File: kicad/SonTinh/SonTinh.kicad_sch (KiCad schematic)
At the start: 11 parts, among them J10 1985195, J11 Conn_01x03_Socket, J12 1985195, J13 Conn_01x03_Socket, J3 Conn_02x03_Odd_Even, J4 1985218, J5 1985218, J7 1985195, J8 1985195

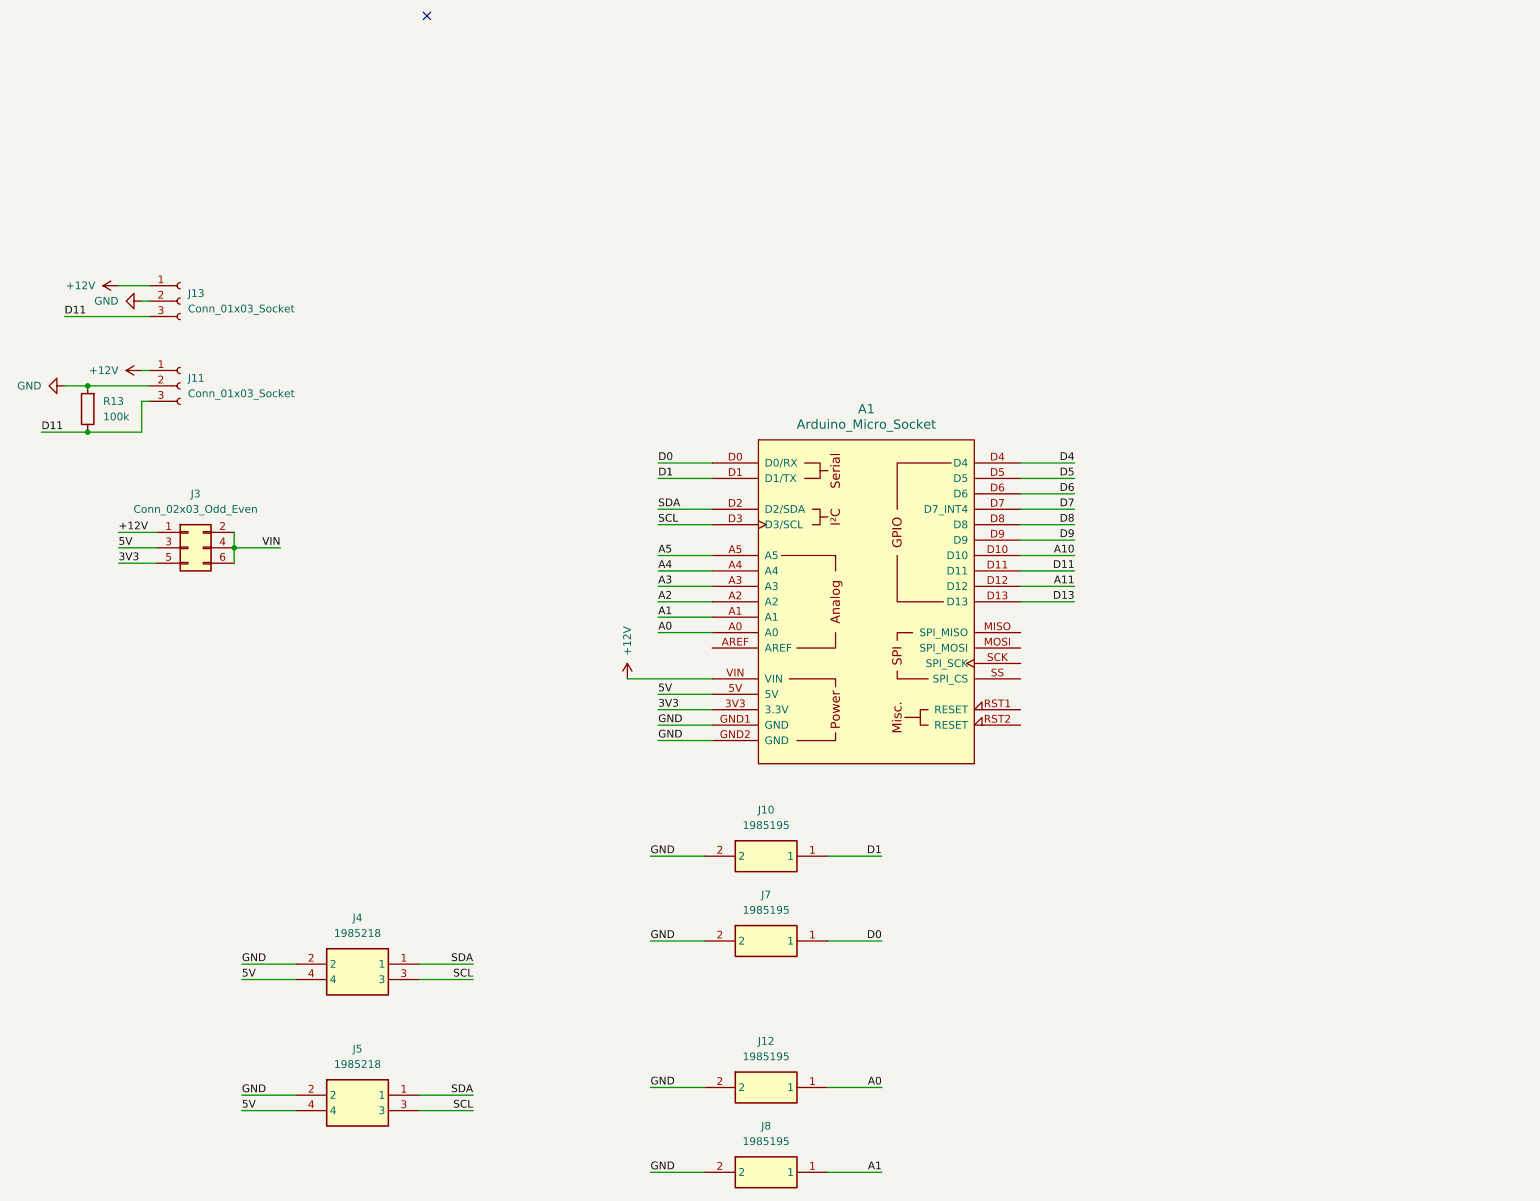
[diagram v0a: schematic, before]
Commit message: The Quill Is Mightier…
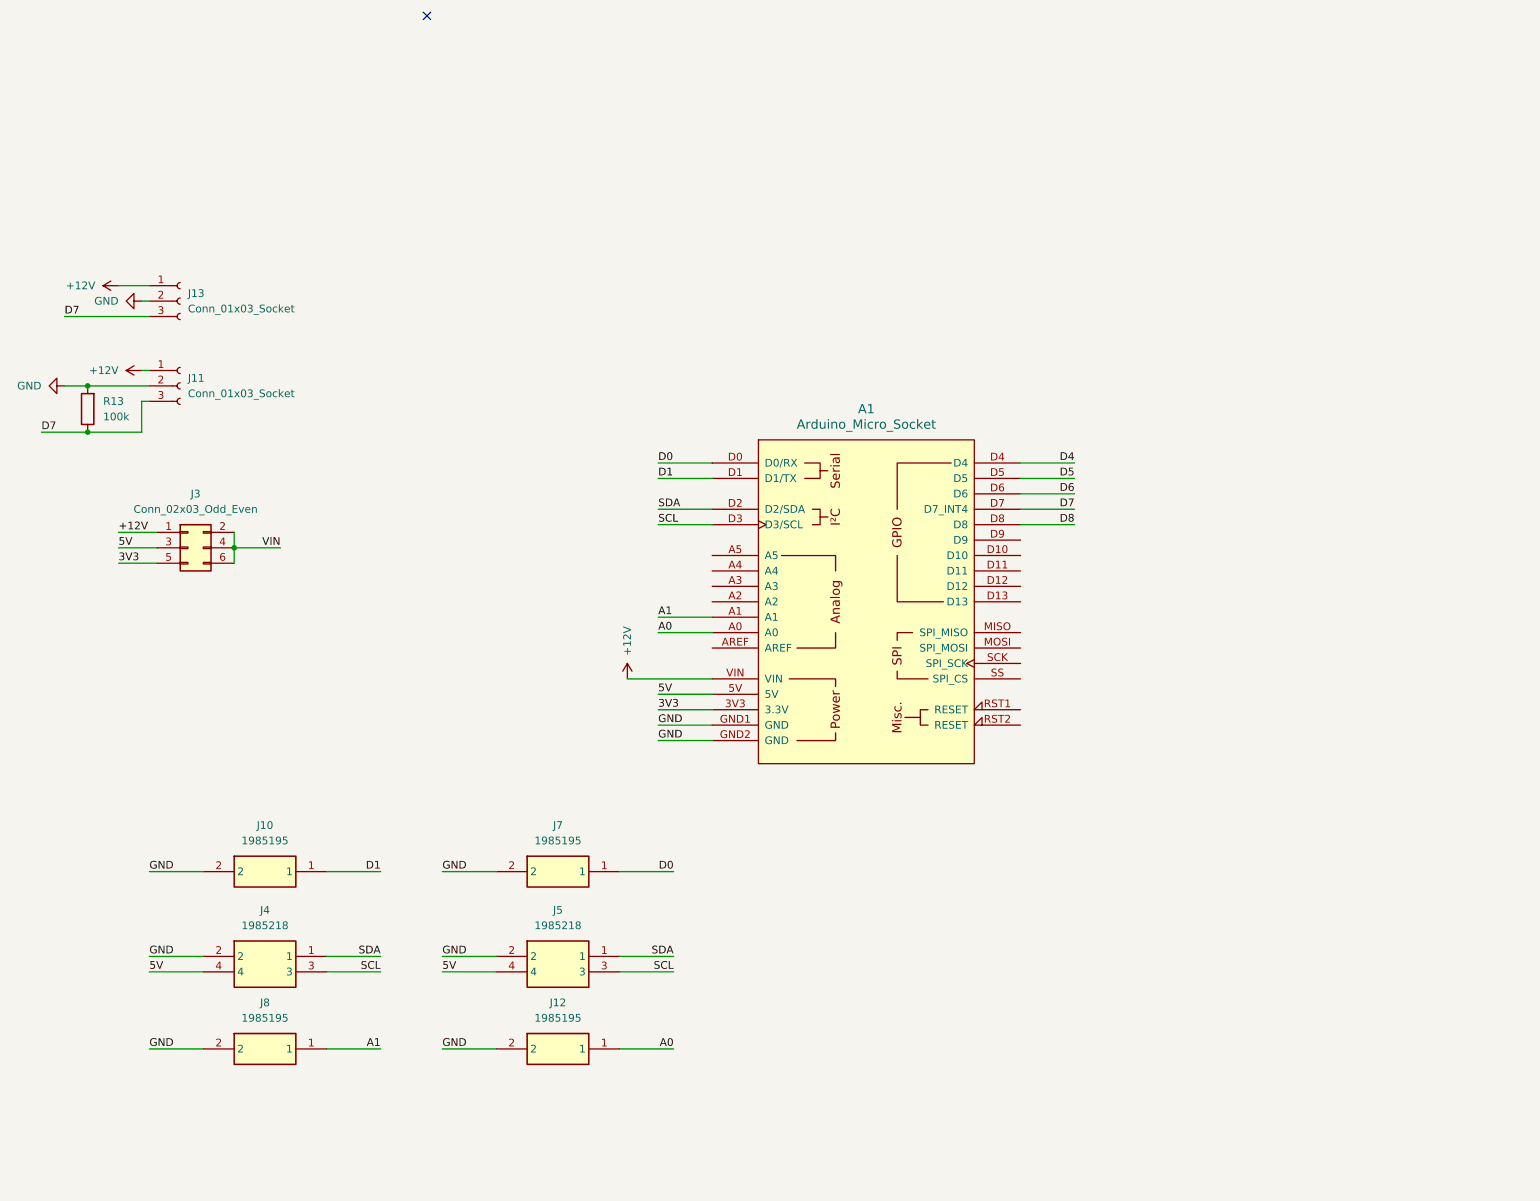
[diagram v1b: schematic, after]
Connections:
- net D7: now also J11.3 (Pin_3), J13.3 (Pin_3), R13.1
- net A10: no longer names the net of A1.D10
- net A11: no longer names the net of A1.D12
- net A2: no longer names the net of A1.A2
- net A3: no longer names the net of A1.A3
- net A4: no longer names the net of A1.A4
- net A5: no longer names the net of A1.A5
- removed net D11: A1.D11, J11.3 (Pin_3), J13.3 (Pin_3), R13.1
- net D13: no longer names the net of A1.D13
- net D9: no longer names the net of A1.D9
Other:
- moved on the sheet: J10, J12, J4, J5, J7, J8

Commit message: The Bitter Suite
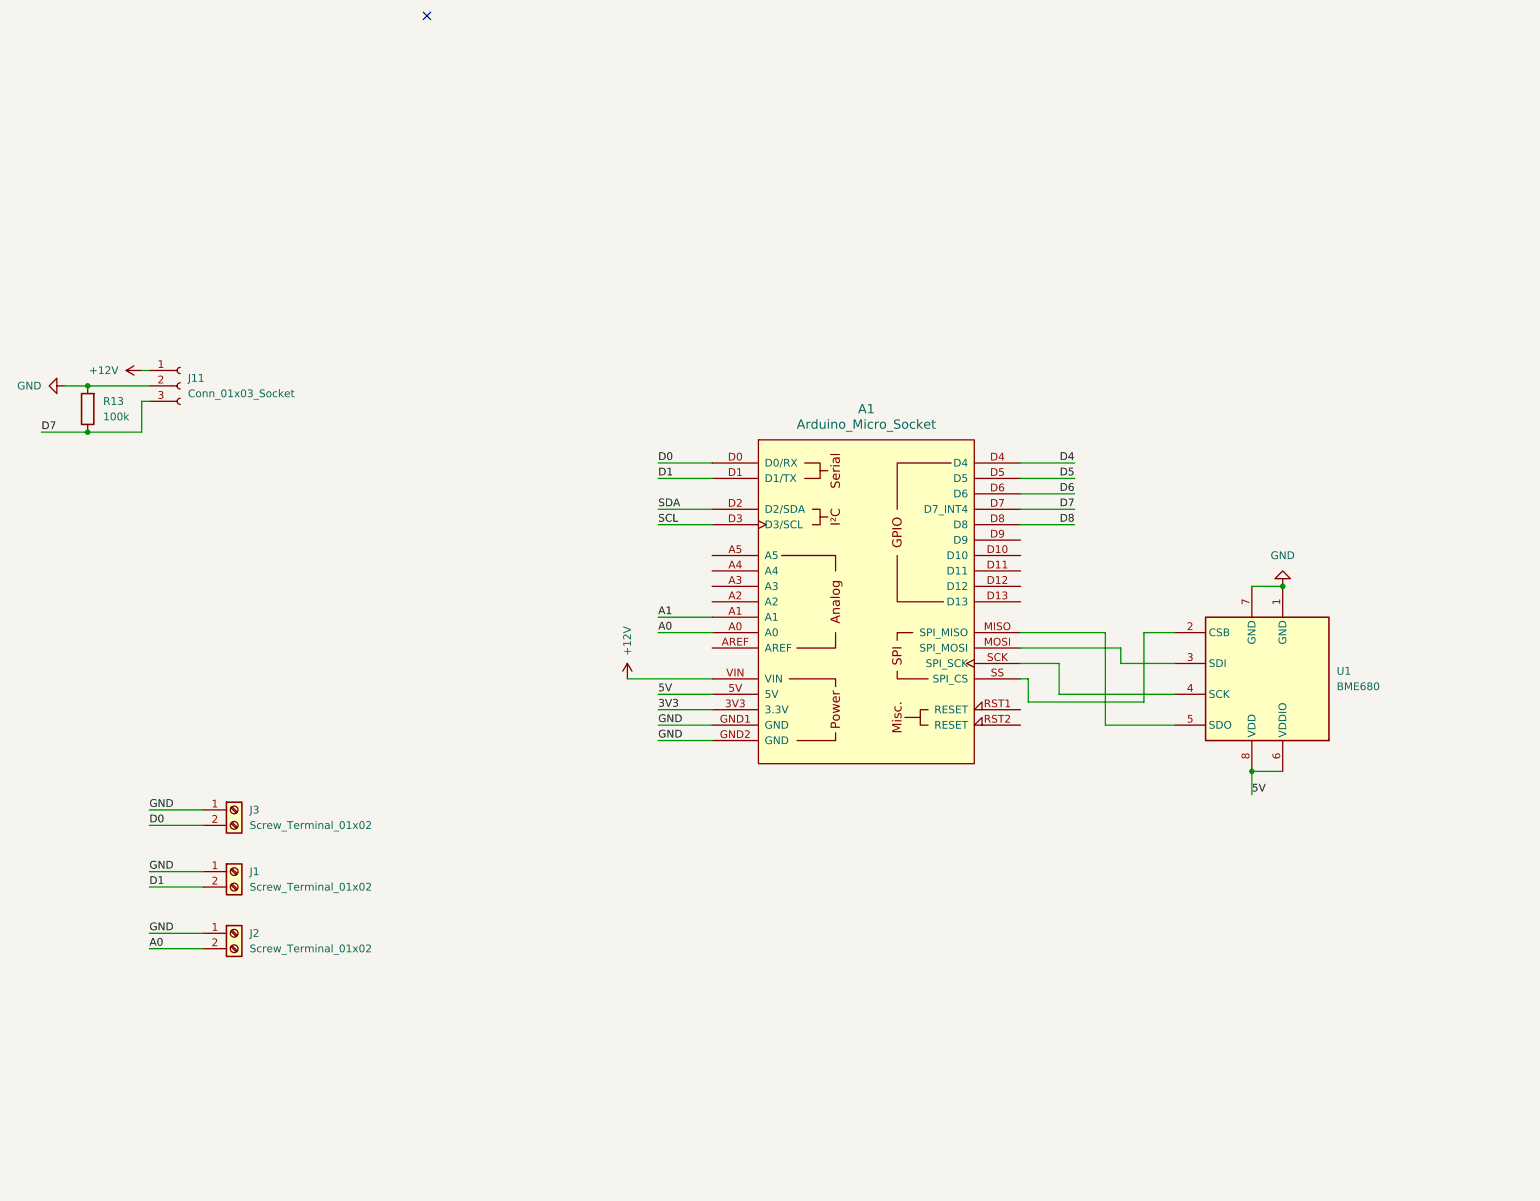
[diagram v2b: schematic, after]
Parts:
- removed J10, J12, J7, J8: 1985195, footprints:1985195, symbol PheonixContact:1985195
- removed J13: Conn_01x03_Socket, Connector_Wire:SolderWire-0.25sqmm_1x03_P4.5mm_D0.65mm_OD2mm, symbol Connector:Conn_01x03_Socket
- removed J3: Conn_02x03_Odd_Even, Connector_PinHeader_2.54mm:PinHeader_2x03_P2.54mm_Vertical, symbol Connector_Generic:Conn_02x03_Odd_Even
- removed J4, J5: 1985218, footprints:PTSA_15_4_35_Z, symbol PheonixContact:1985218
- added J1, J2, J3: Screw_Terminal_01x02, TerminalBlock_Phoenix:TerminalBlock_Phoenix_MPT-0,5-2-2.54_1x02_P2.54mm_Horizontal, symbol Connector:Screw_Terminal_01x02
- added U1: BME680, Package_LGA:Bosch_LGA-8_3x3mm_P0.8mm_ClockwisePinNumbering, symbol Sensor:BME680
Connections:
- net 5V: now also U1.6 (VDDIO), U1.8 (VDD)
- net A0: now also J2.2 (Pin_2)
- net D0: now also J3.2 (Pin_2)
- net D1: now also J1.2 (Pin_2)
- net GND: now also J1.1 (Pin_1), J2.1 (Pin_1), J3.1 (Pin_1), U1.1 (GND), U1.7 (GND)
- net at A1.MISO (SPI_MISO): now also U1.5 (SDO)
- net at A1.MOSI (SPI_MOSI): now also U1.3 (SDI)
- net at A1.SCK (SPI_SCK): now also U1.4 (SCK)
- net at A1.SS (SPI_CS): now also U1.2 (CSB)

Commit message: The Reckoning
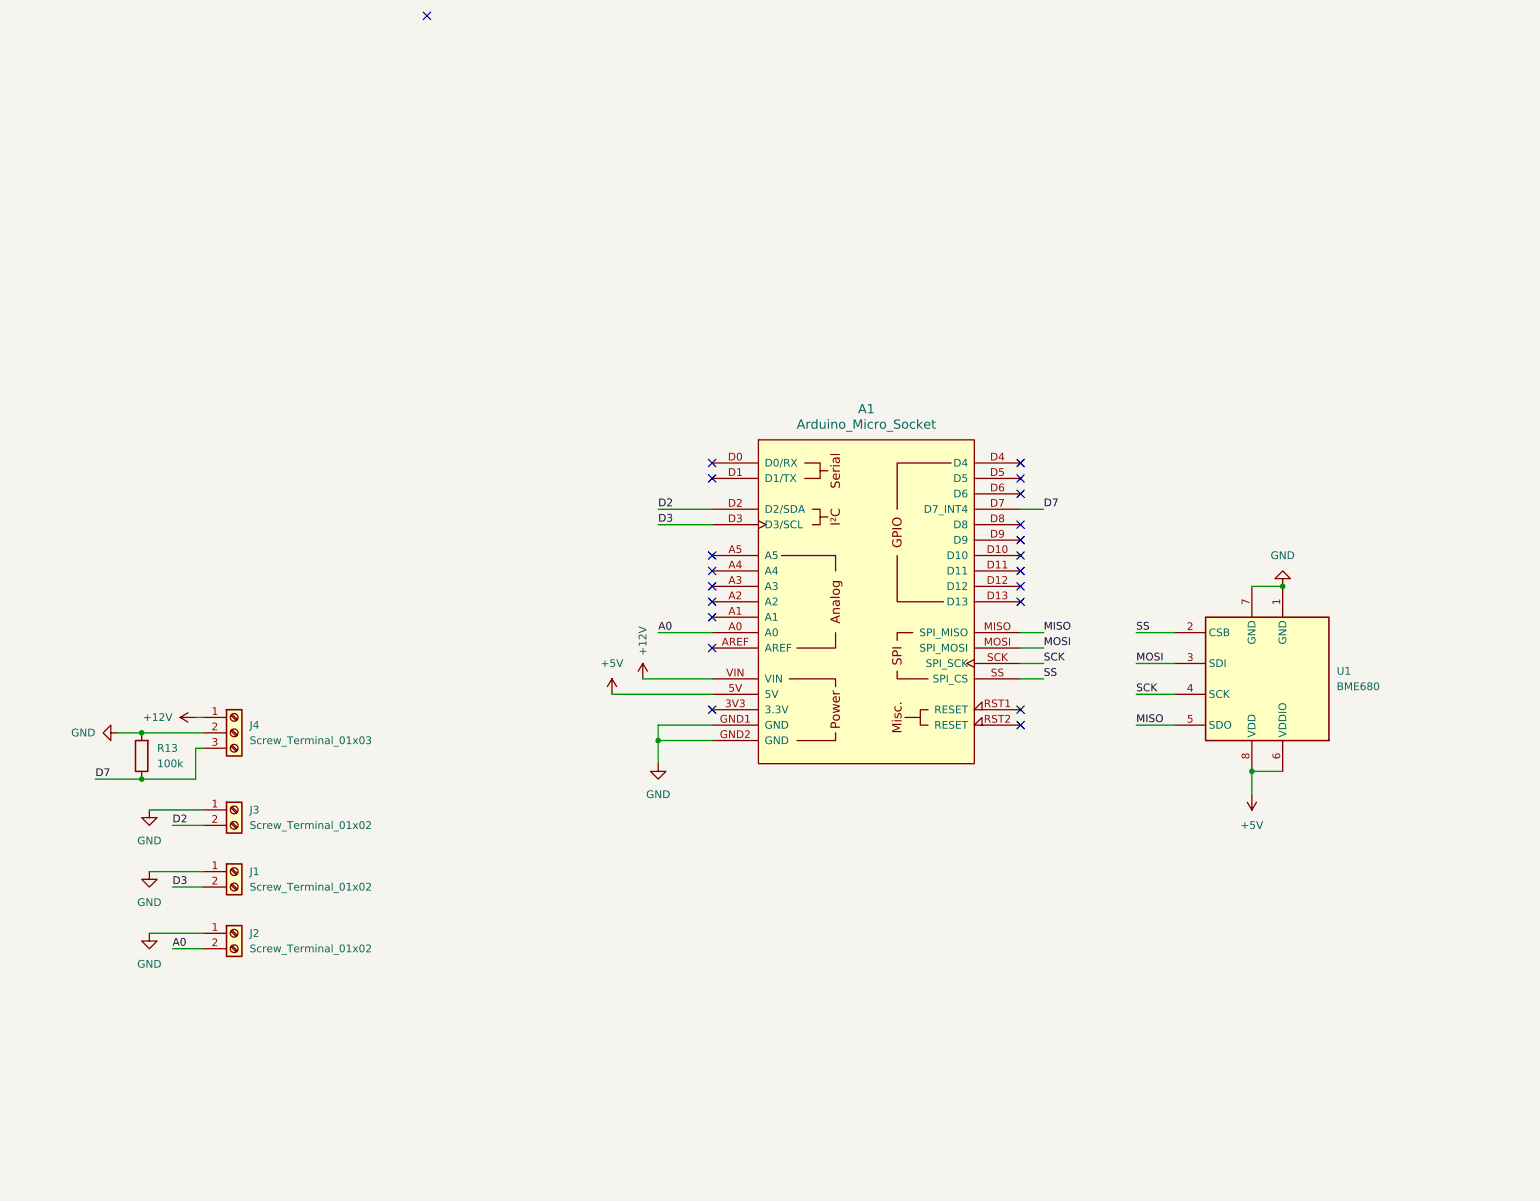
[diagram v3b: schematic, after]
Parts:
- removed J11: Conn_01x03_Socket, Connector_Wire:SolderWire-0.25sqmm_1x03_P4.5mm_D0.65mm_OD2mm, symbol Connector:Conn_01x03_Socket
- added J4: Screw_Terminal_01x03, TerminalBlock_Phoenix:TerminalBlock_Phoenix_MPT-0,5-3-2.54_1x03_P2.54mm_Horizontal, symbol Connector:Screw_Terminal_01x03
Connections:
- net +12V: now also J4.1 (Pin_1)
- net D7: now also J4.3 (Pin_3)
- net GND: now also J4.2 (Pin_2)
- net MISO: now reaches A1.MISO (SPI_MISO), U1.5 (SDO)
- net MOSI: now reaches A1.MOSI (SPI_MOSI), U1.3 (SDI)
- net SCK: now reaches A1.SCK (SPI_SCK), U1.4 (SCK)
- net SS: now reaches A1.SS (SPI_CS), U1.2 (CSB)
- net 3V3: no longer names the net of A1.3V3 (3.3V)
- net 5V renamed +5V
- net A1: no longer names the net of A1.A1
- net D0: no longer names the net of A1.D0 (D0/RX)
- net D0: no longer J3.2 (Pin_2)
- net D1: no longer names the net of A1.D1 (D1/TX)
- net D1: no longer J1.2 (Pin_2)
- net D4: no longer names the net of A1.D4
- net D5: no longer names the net of A1.D5
- net D6: no longer names the net of A1.D6
- net D8: no longer names the net of A1.D8
- net SCL renamed D3
- net D3: now also J1.2 (Pin_2)
- net SDA renamed D2
- net D2: now also J3.2 (Pin_2)
- no-connect marks 1 -> 21
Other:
- moved on the sheet: R13
